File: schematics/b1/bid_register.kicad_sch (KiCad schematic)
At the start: 19 parts, among them SW5 SW_DIP_x08, U5 74HC165

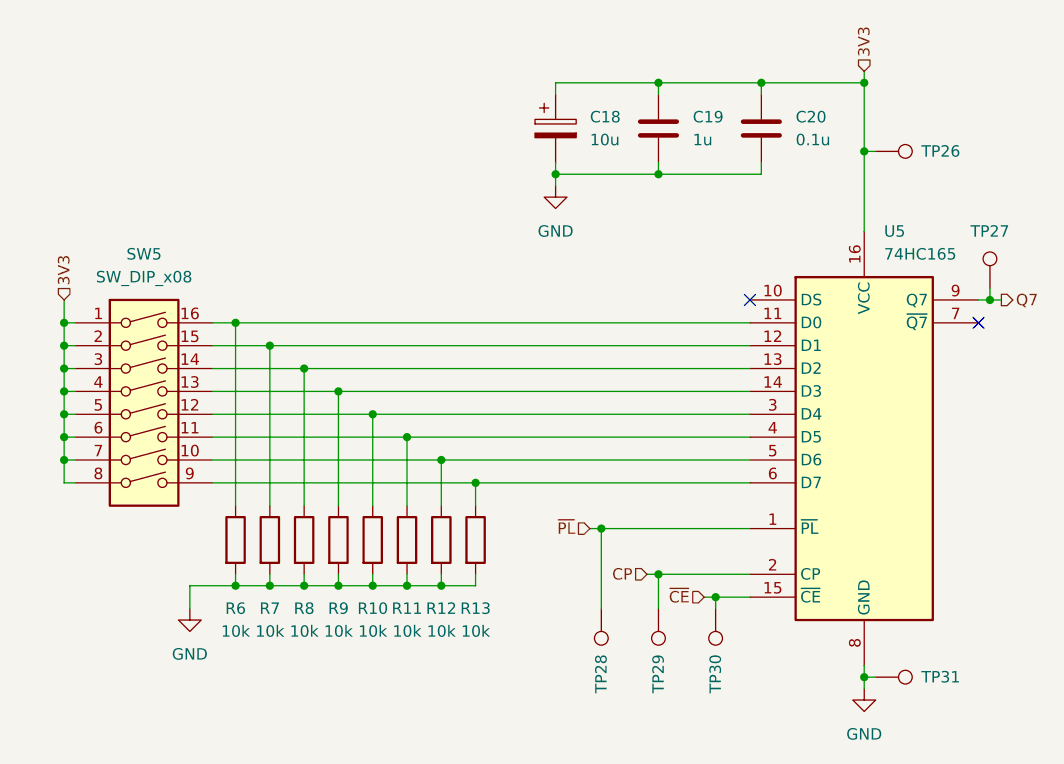
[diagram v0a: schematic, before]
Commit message: Finalizing touches to the B1 schematic.
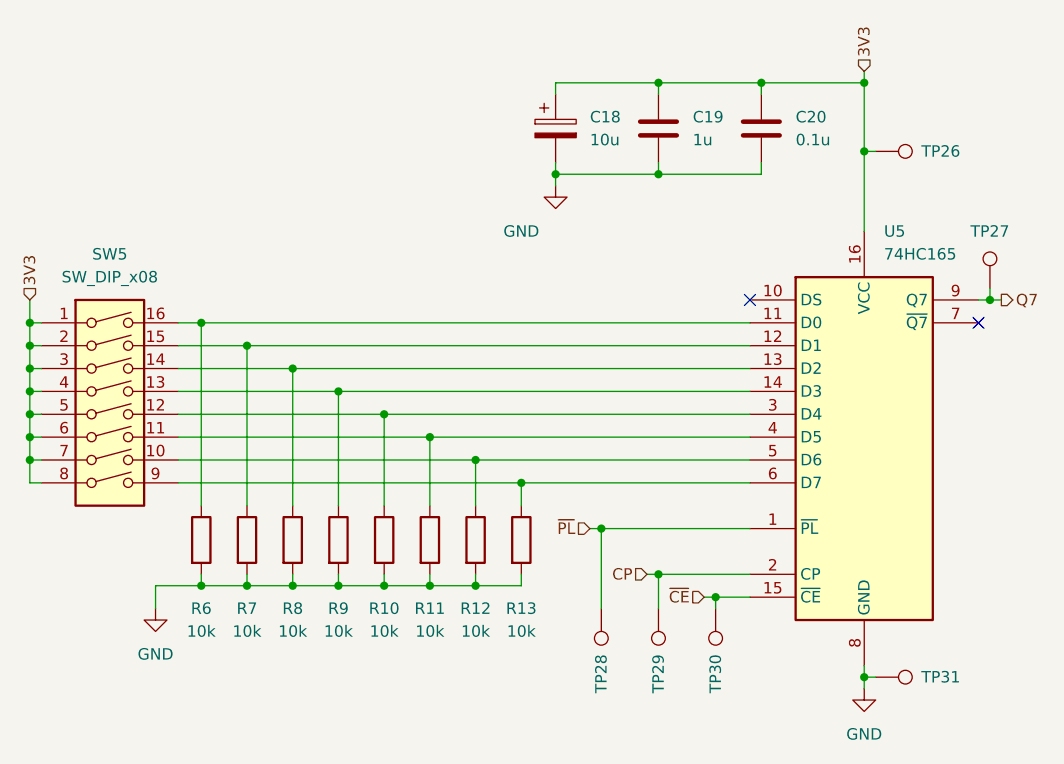
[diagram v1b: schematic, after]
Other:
- moved on the sheet: R10, R11, R12, R13, R6, R7, R8, SW5
